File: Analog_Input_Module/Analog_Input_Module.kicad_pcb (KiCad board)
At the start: 2 copper layers, 60 x 22 mm, 63 parts, among them J1 Conn_02x20_Odd_Even, U1 10K, U10 1.5K, U11 MCP6004, U12 10K, U13 10K, U14 10nF, U15 10nF, U16 MCP6004, U17 1K, U18 1K, U19 1.5K, U2 10K, U20 1.5K, U3 10nF, U4 10nF, U5 MCP6004, U6 MCP6004, U7 1K, U8 1K, U9 1.5K

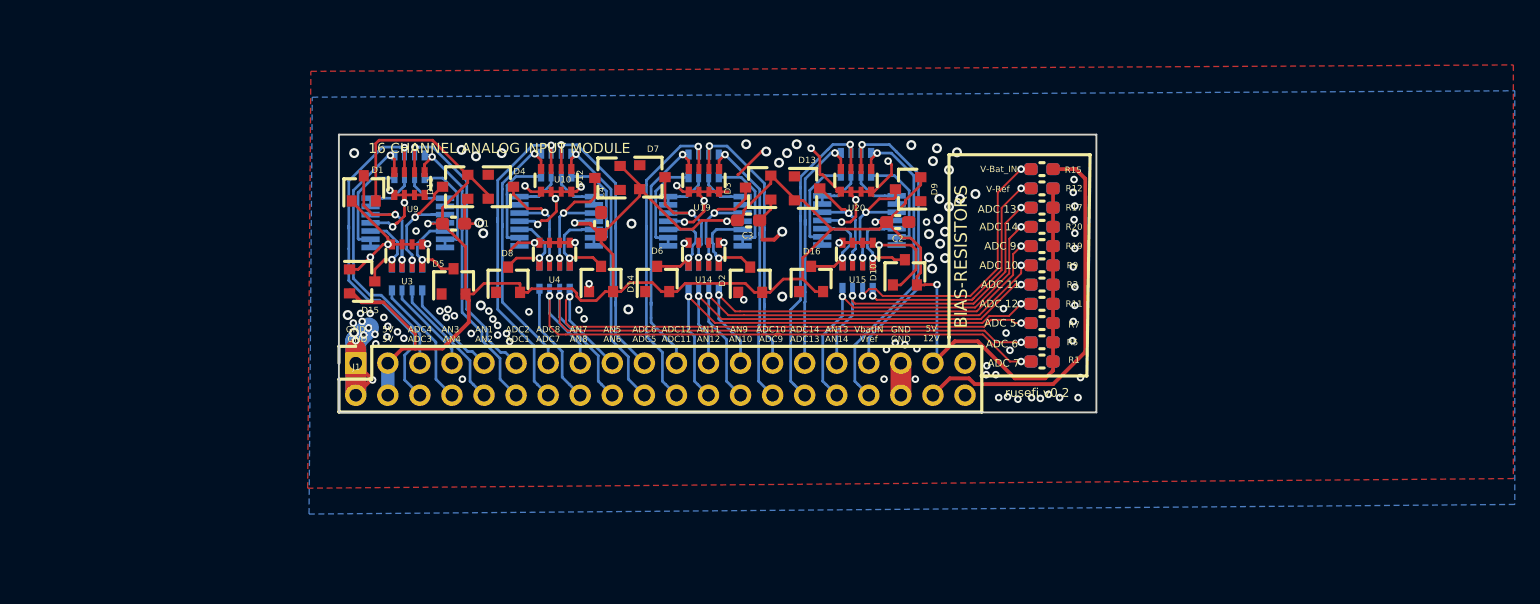
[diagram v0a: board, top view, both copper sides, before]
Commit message: V 0.3 (#30)
* gerbers

* version

* V 0.3
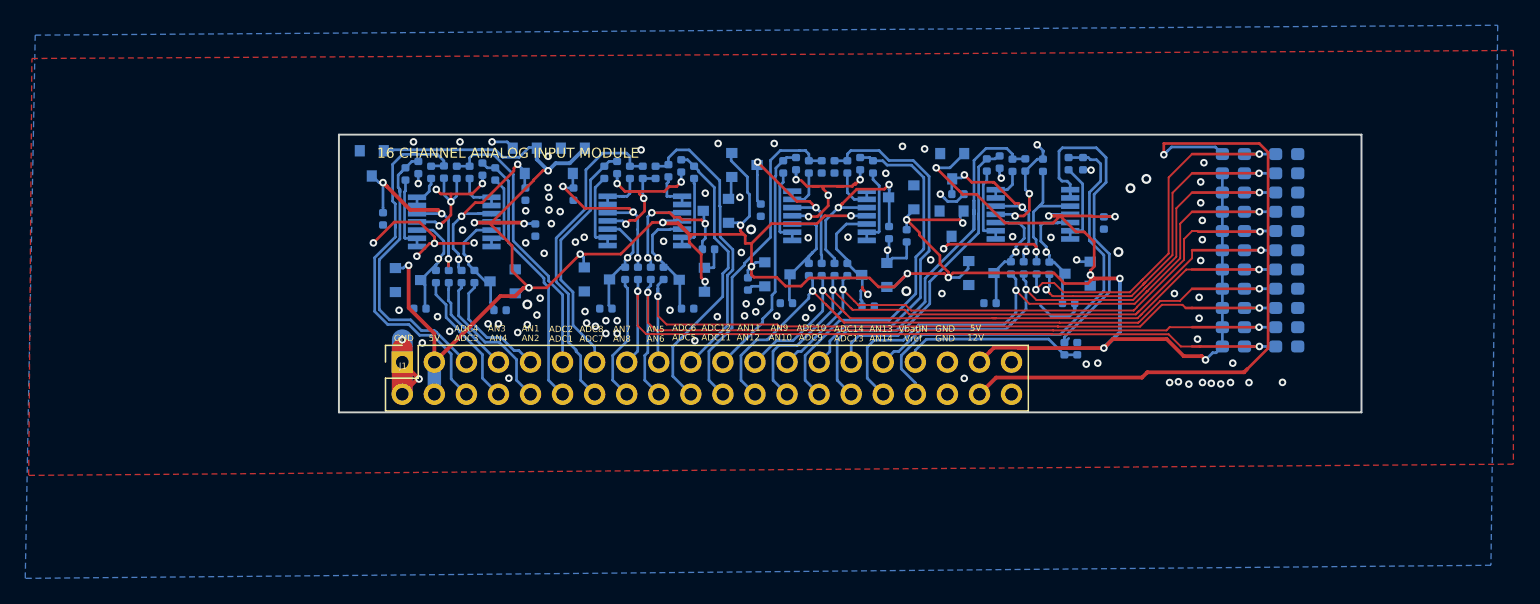
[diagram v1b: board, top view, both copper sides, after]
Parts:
- removed U1, U12, U13, U2: 10K, Resistor_SMD:R_Array_Convex_4x0603
- removed U10, U19, U20, U9: 1.5K, Resistor_SMD:R_Array_Convex_4x0603
- removed U14, U15, U3, U4: 10nF, Resistor_SMD:R_Array_Convex_4x0603
- removed U17, U18, U7, U8: 1K, Resistor_SMD:R_Array_Convex_4x0603
- added C10: 10nF, Capacitor_SMD:C_0402_1005Metric, B.Cu at (49.3, 29.1)
- added C11: 10nF, Capacitor_SMD:C_0402_1005Metric, B.Cu at (38.6, 24.7)
- added C12: 10nF, Capacitor_SMD:C_0402_1005Metric, B.Cu at (41.1, 33.8)
- added C13: 10nF, Capacitor_SMD:C_0402_1005Metric, B.Cu at (77.8, 33.4)
- added C14: 10nF, Capacitor_SMD:C_0402_1005Metric, B.Cu at (61.9, 33.6)
- added C15: 10nF, Capacitor_SMD:C_0402_1005Metric, B.Cu at (75.8, 22.4)
- added C16: 10nF, Capacitor_SMD:C_0402_1005Metric, B.Cu at (63.6, 27.8)
- added C17: 10nF, Capacitor_SMD:C_0402_1005Metric, B.Cu at (69.0, 24.7)
- added C18: 10nF, Capacitor_SMD:C_0402_1005Metric, B.Cu at (53.4, 26.0)
- added C19: 10nF, Capacitor_SMD:C_0402_1005Metric, B.Cu at (71.6, 33.4)
- added C20: 10nF, Capacitor_SMD:C_0402_1005Metric, B.Cu at (55.4, 33.4)
- added C5: 10nF, Capacitor_SMD:C_0402_1005Metric, B.Cu at (32.8, 33.9)
- added C6: 10nF, Capacitor_SMD:C_0402_1005Metric, B.Cu at (34.8, 24.7)
- added C7: 10nF, Capacitor_SMD:C_0402_1005Metric, B.Cu at (23.5, 26.7)
- added C8: 10nF, Capacitor_SMD:C_0402_1005Metric, B.Cu at (26.4, 33.8)
- added C9: 10nF, Capacitor_SMD:C_0402_1005Metric, B.Cu at (47.6, 33.8)
- added R23: 1.5K, Capacitor_SMD:C_0402_1005Metric, B.Cu at (62.3, 22.6)
- added R24: 1.5K, Capacitor_SMD:C_0402_1005Metric, B.Cu at (60.3, 22.6)
- added R25: 1.5K, Capacitor_SMD:C_0402_1005Metric, B.Cu at (57.2, 22.6)
- added R26: 1.5K, Capacitor_SMD:C_0402_1005Metric, B.Cu at (55.2, 22.6)
- added R27: 1K, Capacitor_SMD:C_0402_1005Metric, B.Cu at (61.3, 22.3)
- added R28: 1K, Capacitor_SMD:C_0402_1005Metric, B.Cu at (59.3, 22.6)
- added R29: 1K, Capacitor_SMD:C_0402_1005Metric, B.Cu at (58.2, 22.6)
- added R30: 1K, Capacitor_SMD:C_0402_1005Metric, B.Cu at (56.2, 22.3)
- added R31: 10K, Capacitor_SMD:C_0402_1005Metric, B.Cu at (45.7, 31.0)
- added R32: 10K, Capacitor_SMD:C_0402_1005Metric, B.Cu at (44.7, 31.0)
- added R33: 10K, Capacitor_SMD:C_0402_1005Metric, B.Cu at (43.7, 31.0)
- added R34: 10K, Capacitor_SMD:C_0402_1005Metric, B.Cu at (42.7, 31.0)
- added R35: 10K, Capacitor_SMD:C_0402_1005Metric, B.Cu at (60.3, 30.7)
- added R36: 10K, Capacitor_SMD:C_0402_1005Metric, B.Cu at (59.3, 30.7)
- added R37: 10K, Capacitor_SMD:C_0402_1005Metric, B.Cu at (58.2, 30.7)
- added R38: 10K, Capacitor_SMD:C_0402_1005Metric, B.Cu at (57.2, 30.7)
- added R39: 10K, Capacitor_SMD:C_0402_1005Metric, B.Cu at (30.7, 31.2)
- added R40: 10K, Capacitor_SMD:C_0402_1005Metric, B.Cu at (29.7, 31.2)
- added R41: 10K, Capacitor_SMD:C_0402_1005Metric, B.Cu at (28.7, 31.2)
- added R42: 10K, Capacitor_SMD:C_0402_1005Metric, B.Cu at (27.7, 31.2)
- added R43: 1.5K, Capacitor_SMD:C_0402_1005Metric, B.Cu at (32.4, 23.1)
- added R44: 1.5K, Capacitor_SMD:C_0402_1005Metric, B.Cu at (30.4, 23.0)
- added R45: 1.5K, Capacitor_SMD:C_0402_1005Metric, B.Cu at (27.3, 23.0)
- added R46: 1.5K, Capacitor_SMD:C_0402_1005Metric, B.Cu at (25.3, 23.1)
- added R47: 1K, Capacitor_SMD:C_0402_1005Metric, B.Cu at (31.4, 22.7)
- added R48: 1K, Capacitor_SMD:C_0402_1005Metric, B.Cu at (29.3, 23.0)
- added R49: 1K, Capacitor_SMD:C_0402_1005Metric, B.Cu at (28.3, 23.0)
- added R50: 1K, Capacitor_SMD:C_0402_1005Metric, B.Cu at (26.3, 22.6)
- added R51: 1.5K, Capacitor_SMD:C_0402_1005Metric, B.Cu at (48.1, 23.0)
- added R52: 1.5K, Capacitor_SMD:C_0402_1005Metric, B.Cu at (46.1, 22.9)
- added R53: 1.5K, Capacitor_SMD:C_0402_1005Metric, B.Cu at (43.1, 23.0)
- added R54: 1.5K, Capacitor_SMD:C_0402_1005Metric, B.Cu at (41.0, 23.0)
- added R55: 1K, Capacitor_SMD:C_0402_1005Metric, B.Cu at (47.1, 22.5)
- added R56: 1K, Capacitor_SMD:C_0402_1005Metric, B.Cu at (45.1, 23.0)
- added R57: 1K, Capacitor_SMD:C_0402_1005Metric, B.Cu at (44.1, 23.0)
- added R58: 1K, Capacitor_SMD:C_0402_1005Metric, B.Cu at (42.0, 22.6)
- added R59: 10K, Capacitor_SMD:C_0402_1005Metric, B.Cu at (76.3, 30.6)
- added R60: 10K, Capacitor_SMD:C_0402_1005Metric, B.Cu at (75.3, 30.6)
- added R61: 10K, Capacitor_SMD:C_0402_1005Metric, B.Cu at (74.2, 30.6)
- added R62: 10K, Capacitor_SMD:C_0402_1005Metric, B.Cu at (73.2, 30.6)
- added R63: 1.5K, Capacitor_SMD:C_0402_1005Metric, B.Cu at (77.8, 22.3)
- added R64: 1.5K, Capacitor_SMD:C_0402_1005Metric, B.Cu at (77.5, 37.0)
- added R65: 1.5K, Capacitor_SMD:C_0402_1005Metric, B.Cu at (73.4, 22.4)
- added R66: 1.5K, Capacitor_SMD:C_0402_1005Metric, B.Cu at (71.3, 22.4)
- added R67: 1K, Capacitor_SMD:C_0402_1005Metric, B.Cu at (78.9, 22.3)
- added R68: 1K, Capacitor_SMD:C_0402_1005Metric, B.Cu at (78.5, 37.0)
- added R69: 1K, Capacitor_SMD:C_0402_1005Metric, B.Cu at (74.4, 22.4)
- added R70: 1K, Capacitor_SMD:C_0402_1005Metric, B.Cu at (72.3, 22.2)
- C1, C2, C3, C4: value 0.1uF -> 100nF; footprint Capacitor_SMD:C_0603_1608Metric_Pad1.05x0.95mm_HandSolder -> Capacitor_SMD:C_0402_1005Metric; moved to B.Cu
- D1, D10, D11, D12, D13, D14, D15, D16, D2, D3, D4, D5, D6, D7, D8, D9, R1, R11, R12, R15, R17, R19, R2, R20, R5, R7, R9: moved to B.Cu
- moved R10 19.4 mm to (95.1, 29.2)
- moved R13 19.4 mm to (95.1, 32.2)
- moved R14 19.4 mm to (95.1, 23.1)
- moved R16 19.4 mm to (95.1, 21.5)
- moved R18 19.4 mm to (95.1, 24.6)
- moved R21 19.4 mm to (95.1, 27.6)
- moved R22 19.4 mm to (95.1, 26.1)
- moved R3 19.4 mm to (95.1, 36.8)
- moved R4 19.4 mm to (95.1, 30.7)
- moved R6 19.4 mm to (95.1, 35.3)
- moved R8 19.4 mm to (95.1, 33.7)
- moved C2 16.3 mm to (80.6, 27.0), turned to 270 degrees
- moved R1 15.2 mm to (90.9, 36.8), turned to 180 degrees
- moved R11 15.2 mm to (90.9, 32.2), turned to 180 degrees
- moved R12 15.2 mm to (90.9, 23.1), turned to 180 degrees
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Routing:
- net /5V: track 179.8 -> 239.6 mm, vias 5 -> 22
- net /U-Batt: track 30.4 -> 54.5 mm, vias 0 -> 1
- net Net-(R64-Pad2): track 4.50 -> 26.0 mm
- net /ADC_14: track 29.9 -> 47.4 mm
- net /ADC_12: track 38.6 -> 55.0 mm
- net /ADC_13: track 27.3 -> 43.6 mm
- net /ADC_10: track 38.4 -> 52.6 mm
- net /ADC_11: track 36.4 -> 50.5 mm
- net /ADC_9: track 35.7 -> 48.9 mm
- net /ADC_7: track 49.8 -> 62.4 mm
- net /ADC_6: track 51.1 -> 63.7 mm
- net /ADC_5: track 47.9 -> 60.2 mm
- net /U-Batt_MCU: track 24.8 -> 14.7 mm, vias 1 -> 0
- net /Vref: track 25.4 -> 35.4 mm, vias 1 -> 0
- net Net-(C15-Pad1): track 11.0 -> 19.4 mm
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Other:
- board size 60 x 22 mm -> 81 x 22 mm
- board text added: "rusefi v0.3"
- board text removed: "rusefi v0.2"
